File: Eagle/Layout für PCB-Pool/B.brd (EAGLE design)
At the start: 56.5 x 20.3 mm, 17 parts, among them IC1 78L05, IC2 MAX3232CPE

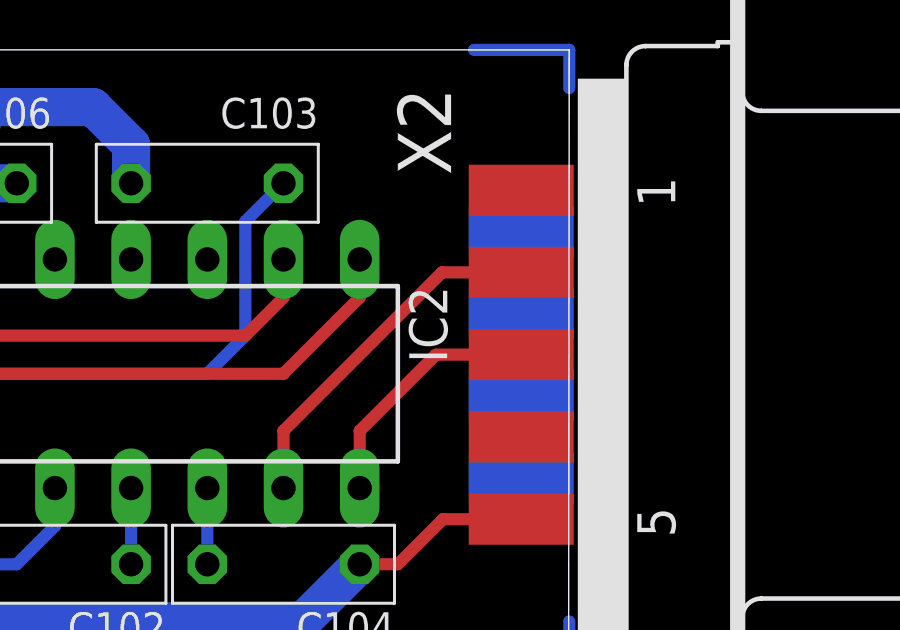
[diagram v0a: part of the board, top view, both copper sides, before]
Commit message: SWE: Nutzen für PCB-Pool
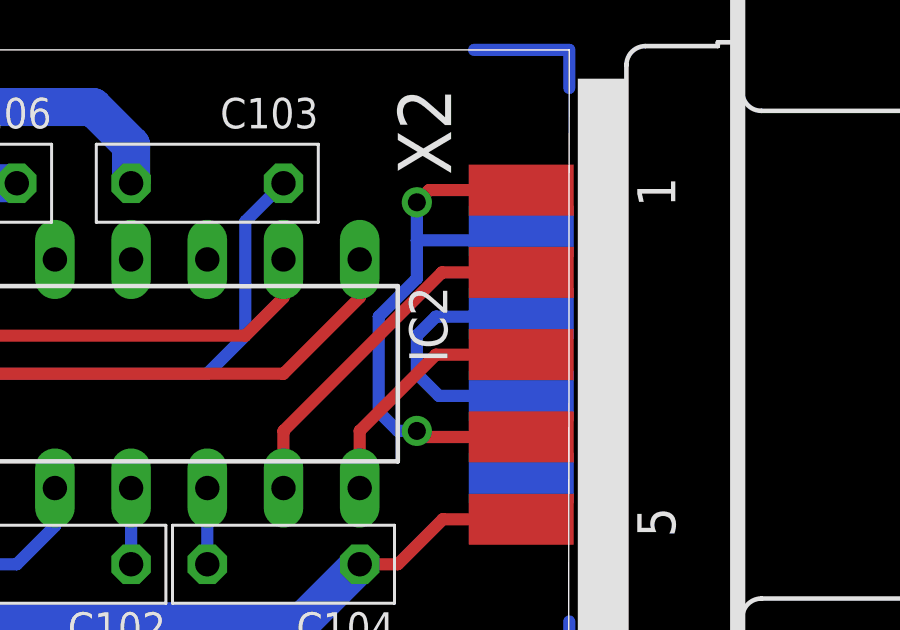
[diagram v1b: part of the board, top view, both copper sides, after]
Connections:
- new net N$2: X2.7, X2.8
- new net N$3: X2.1, X2.4, X2.6
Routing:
- net N$3: track 0.00 -> 20.0 mm, vias 0 -> 2
- net N$2: track 0.00 -> 8.84 mm
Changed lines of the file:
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@@
 <setting verticaltext="up"/>
 </settings>
-<grid distance="0.025" unitdist="inch" unit="inch" style="lines" multiple="1" display="yes" altdistance="0.025" altunitdist="inch" altunit="inch"/>
+<grid distance="0.025" unitdist="inch" unit="mm" style="lines" multiple="1" display="yes" altdistance="0.025" altunitdist="inch" altunit="inch"/>
 <layers>
 <layer number="1" name="Top" color="4" fill="1" visible="yes" active="yes"/>
@@
 <wire x1="36.195" y1="1.27" x2="36.195" y2="0" width="0.4064" layer="16"/>
 </signal>
+<signal name="N$2">
+<contactref element="X2" pad="8"/>
+<contactref element="X2" pad="7"/>
+<wire x1="34.5948" y1="8.7884" x2="31.8516" y2="8.7884" width="0.4064" layer="16"/>
+<wire x1="31.8516" y1="8.7884" x2="31.115" y2="9.525" width="0.4064" layer="16"/>
+<wire x1="31.115" y1="9.525" x2="31.115" y2="10.795" width="0.4064" layer="16"/>
+<wire x1="31.115" y1="10.795" x2="31.75" y2="11.43" width="0.4064" layer="16"/>
+<wire x1="31.75" y1="11.43" x2="34.4932" y2="11.43" width="0.4064" layer="16"/>
+<wire x1="34.4932" y1="11.43" x2="34.5948" y2="11.5316" width="0.4064" layer="16"/>
+</signal>
+<signal name="N$3">
+<contactref element="X2" pad="6"/>
+<contactref element="X2" pad="4"/>
+<contactref element="X2" pad="1"/>
+<wire x1="34.5952" y1="7.4166" x2="31.115" y2="7.4166" width="0.4064" layer="1"/>
+<wire x1="31.115" y1="7.4166" x2="31.115" y2="7.62" width="0.4064" layer="1"/>
+<via x="31.115" y="7.62" extent="1-16" drill="0.6"/>
+<wire x1="31.115" y1="7.62" x2="30.48" y2="7.62" width="0.4064" layer="16"/>
+<wire x1="30.48" y1="7.62" x2="29.845" y2="8.255" width="0.4064" layer="16"/>
+<wire x1="29.845" y1="8.255" x2="29.845" y2="11.43" width="0.4064" layer="16"/>
+<wire x1="29.845" y1="11.43" x2="31.115" y2="12.7" width="0.4064" layer="16"/>
+<wire x1="31.115" y1="12.7" x2="31.115" y2="13.97" width="0.4064" layer="16"/>
+<wire x1="31.115" y1="13.97" x2="34.29" y2="13.97" width="0.4064" layer="16"/>
+<wire x1="34.29" y1="13.97" x2="34.5948" y2="14.2748" width="0.4064" layer="16"/>
+<wire x1="34.5952" y1="15.6462" x2="31.5212" y2="15.6462" width="0.4064" layer="1"/>
+<wire x1="31.5212" y1="15.6462" x2="31.115" y2="15.24" width="0.4064" layer="1"/>
+<via x="31.115" y="15.24" extent="1-16" drill="0.6"/>
+<wire x1="31.115" y1="13.97" x2="31.115" y2="15.24" width="0.4064" layer="16"/>
+</signal>
 </signals>
